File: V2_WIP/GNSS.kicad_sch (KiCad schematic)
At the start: 17 parts, among them J301 *USB_B_Micro, U301 USBLC6-2SC6, U401 *NEO-M9N

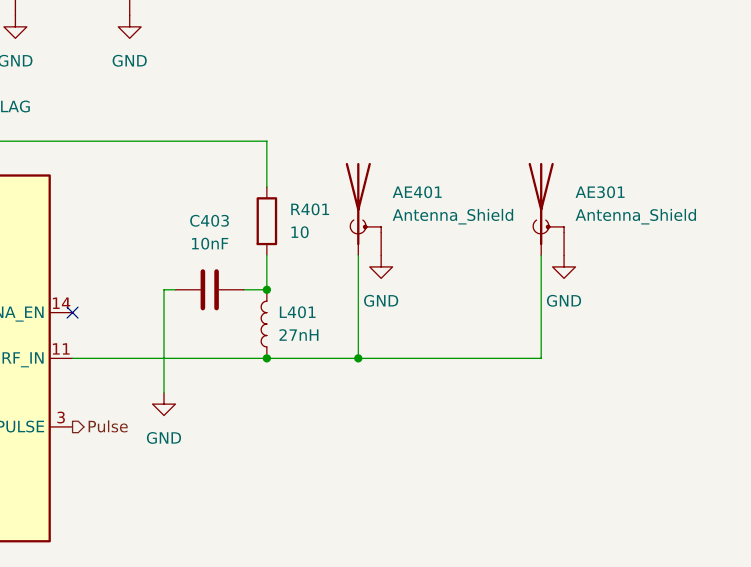
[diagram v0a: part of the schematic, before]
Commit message: up to date i dont remember what changed
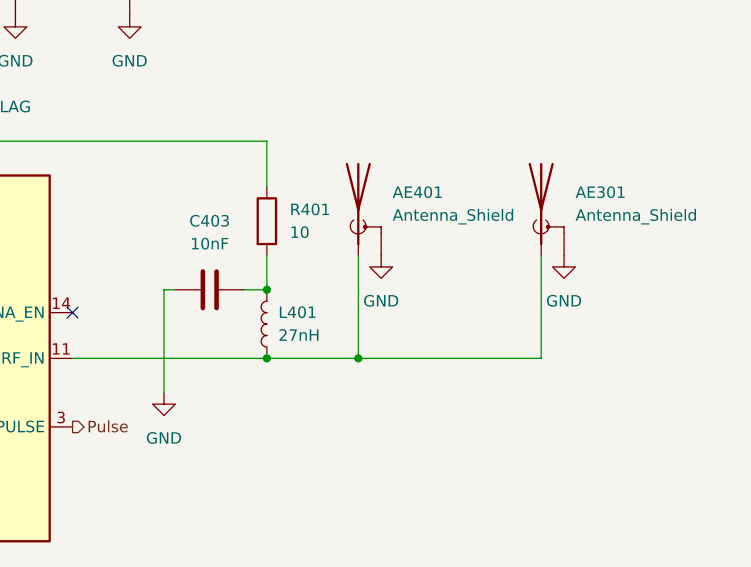
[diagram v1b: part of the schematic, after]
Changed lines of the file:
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@@
 (kicad_sch
-	(version 20231120)
+	(version 20250114)
 	(generator "eeschema")
-	(generator_version "8.0")
+	(generator_version "9.0")
 	(paper "A4")
 	(junction
@@
 		(shape input)
 		(at 111.76 102.87 180)
-		(fields_autoplaced yes)
 		(effects
 			(font
@@
 		(shape output)
 		(at 76.2 77.47 90)
-		(fields_autoplaced yes)
 		(effects
 			(font
@@
 		(shape output)
 		(at 157.48 115.57 0)
-		(fields_autoplaced yes)
 		(effects
 			(font
@@
 		(shape output)
 		(at 111.76 100.33 180)
-		(fields_autoplaced yes)
 		(effects
 			(font
